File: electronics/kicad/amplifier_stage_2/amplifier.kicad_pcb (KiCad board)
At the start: 2 copper layers, 12 parts, among them J1 CONSMA001-SMD-G, U1 BFP620, U2 CE3520K3

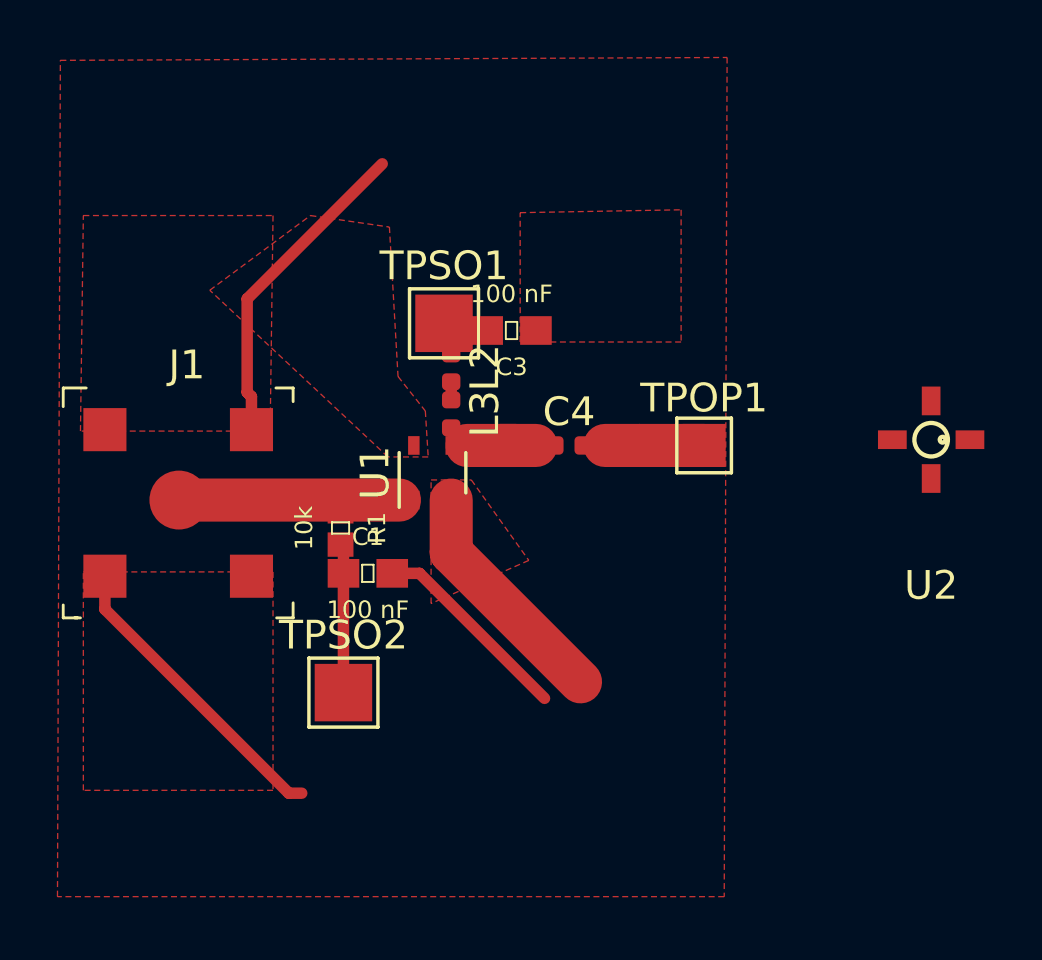
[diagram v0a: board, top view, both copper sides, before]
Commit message: S2 amp
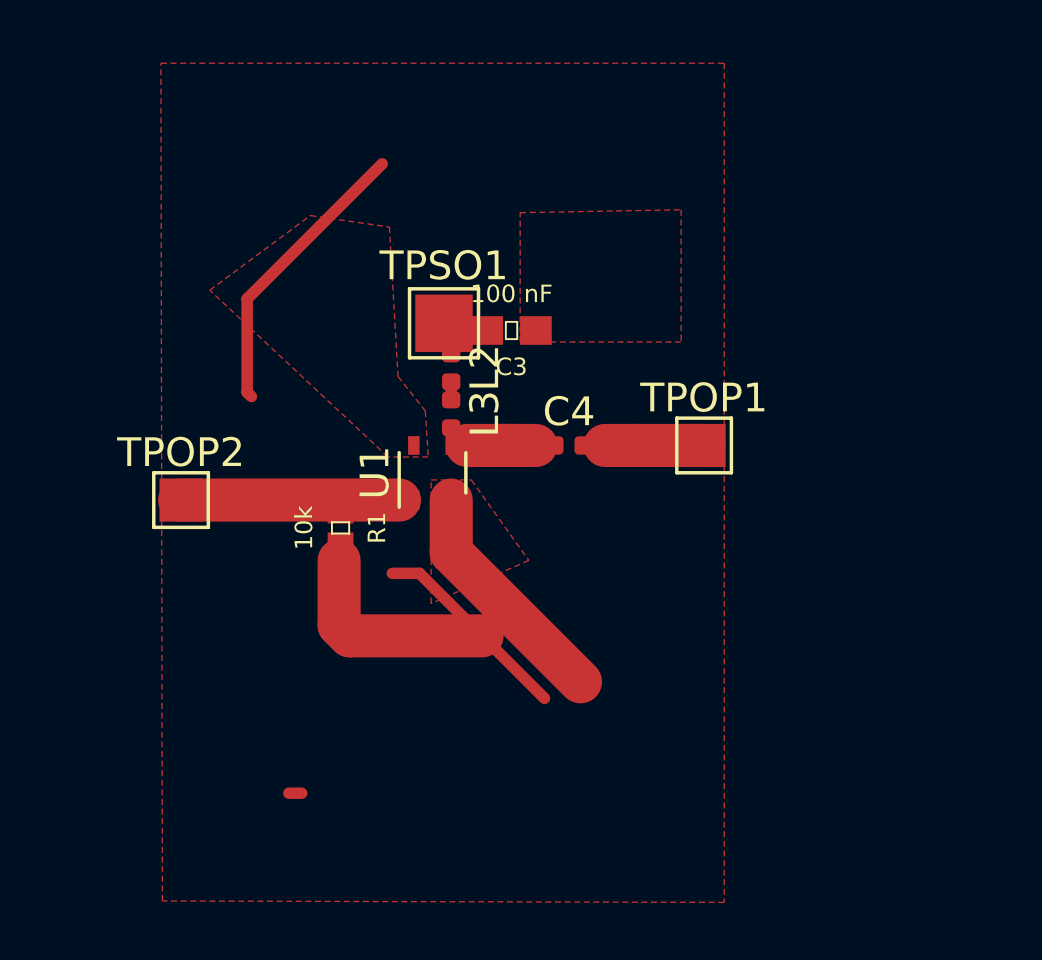
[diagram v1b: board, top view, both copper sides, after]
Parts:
- removed C1: 100 nF, Capacitors:0603
- removed J1: CONSMA001-SMD-G, digikey-footprints:RF_SMA_Receptical_Vertical_CONSMA001-SMD-G
- removed TPSO2: Vsource, TestPoint:TestPoint_Pad_2.0x2.0mm
- removed U2: CE3520K3, 0xDBFB7:4-Micro-X
- added TPOP2: Voutput, TestPoint:TestPoint_Pad_1.5x1.5mm, F.Cu at (141.6, 106.5)
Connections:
- R1 pad 2: Net-(C1-Pad1) -> GND
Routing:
- net Net-(C1-Pad1): track 5.19 -> 0.00 mm
- net GND: track 37.2 -> 34.3 mm
